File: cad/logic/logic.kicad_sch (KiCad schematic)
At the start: 32 parts, among them J1 Conn_01x02, J10 Conn_01x02, J2 Conn_01x02, J3 Conn_01x02, J4 Conn_01x02, J5 Conn_01x02, J6 Conn_01x02, J7 Conn_01x02, J8 Conn_01x02, J9 Conn_01x06, U1 74HC595, U2 TPL7407LAD, U3 TPL7407LAD, U4 TPL7407LAD

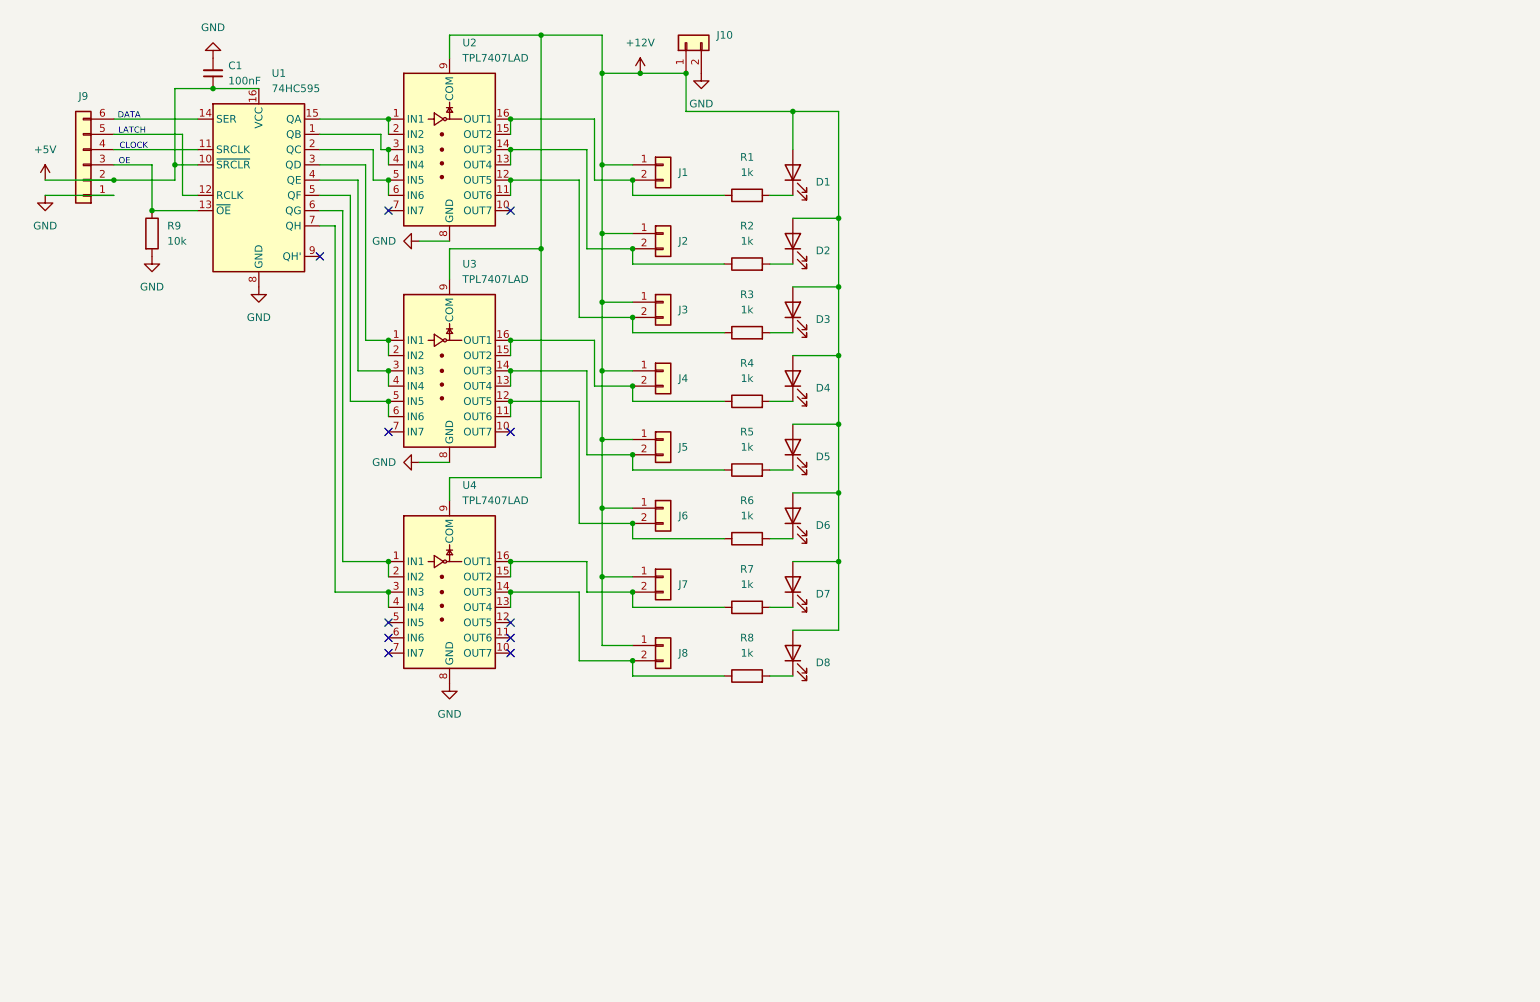
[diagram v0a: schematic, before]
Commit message: Initial design complete
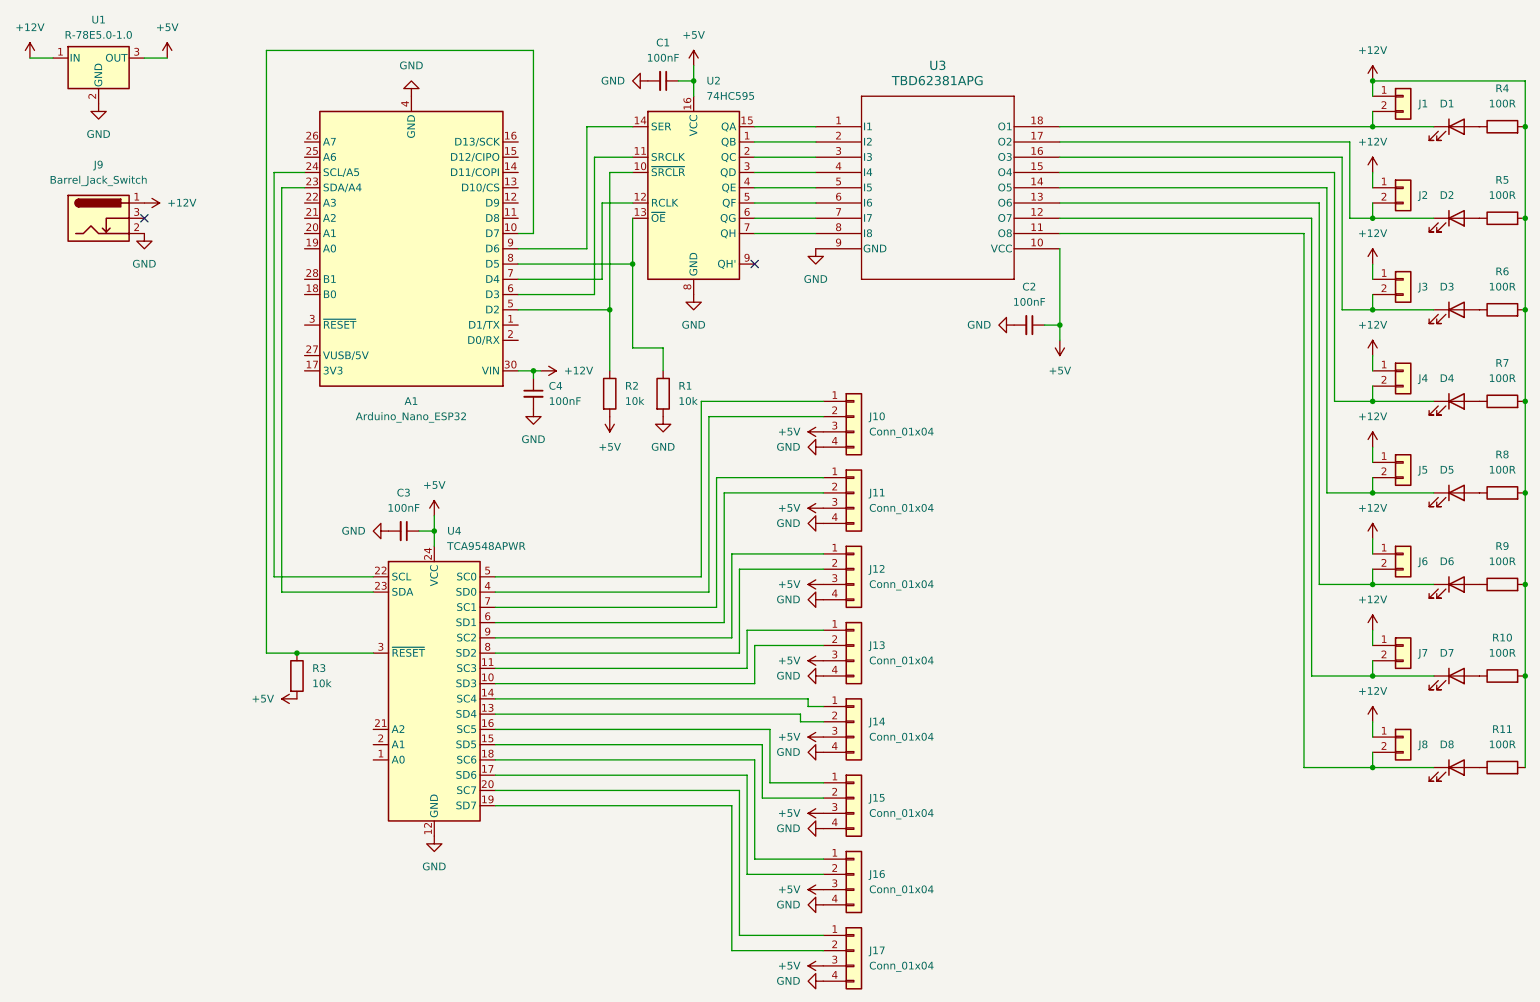
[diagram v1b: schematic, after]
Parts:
- removed J10: Conn_01x02, Connector_JST:JST_PH_B2B-PH-K_1x02_P2.00mm_Vertical, symbol Connector_Generic:Conn_01x02
- removed J9: Conn_01x06, Connector_JST:JST_PH_B6B-PH-K_1x06_P2.00mm_Vertical, symbol Connector_Generic:Conn_01x06
- removed U1: 74HC595, Package_DIP:DIP-16_W7.62mm_Socket, symbol 74xx:74HC595
- removed U2, U3, U4: TPL7407LAD, Package_SO:SOIC-16_3.9x9.9mm_P1.27mm, symbol Transistor_Array:TPL7407LAD
- added A1: Arduino_Nano_ESP32, Module:Arduino_Nano, symbol MCU_Module:Arduino_Nano_ESP32
- added C2, C3, C4: 100nF, Capacitor_THT:C_Disc_D4.7mm_W2.5mm_P5.00mm, symbol Device:C_Small
- added J10, J11, J12, J13, J14, J15, J16, J17: Conn_01x04, Connector_JST:JST_PH_B4B-PH-K_1x04_P2.00mm_Vertical, symbol Connector_Generic:Conn_01x04
- added J9: Barrel_Jack_Switch, Connector_BarrelJack:BarrelJack_Horizontal, symbol Connector:Barrel_Jack_Switch
- added R10, R11: 100R, Resistor_THT:R_Axial_DIN0207_L6.3mm_D2.5mm_P7.62mm_Horizontal, symbol Device:R
- added U1: R-78E5.0-1.0, Converter_DCDC:Converter_DCDC_RECOM_R-78E-0.5_THT, symbol Regulator_Switching:R-78E5.0-1.0
- added U2: 74HC595, Package_DIP:DIP-16_W7.62mm_Socket, symbol 74xx:74HC595
- added U3: TBD62381APG, footprints:P-DIP18-300-2p54-001_TOS, symbol watersystem:TBD62381APG
- added U4: TCA9548APWR, Package_DIP:DIP-24_18.0mmx34.29mm_W15.24mm_Socket, symbol Interface_Expansion:TCA9548APWR
- C1: footprint Capacitor_SMD:C_0805_2012Metric_Pad1.18x1.45mm_HandSolder -> Capacitor_THT:C_Disc_D4.7mm_W2.5mm_P5.00mm
- R1, R2, R3: value 1k -> 10k
- R4, R5, R6, R7, R8: value 1k -> 100R
- R9: value 10k -> 100R
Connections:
- net +12V: now also R4.2, R5.2, R6.2, R7.2, R8.2, R9.2, A1.30 (VIN), C4.1, J9.1, R10.2, R11.2, U1.1 (IN); no longer D1.2 (A), D2.2 (A), D3.2 (A), D4.2 (A), D5.2 (A), D6.2 (A), D7.2 (A), D8.2 (A)
- net +5V: now also R2.2, R3.2, C2.1, C3.1, J10.3 (Pin_3), J11.3 (Pin_3), J12.3 (Pin_3), J13.3 (Pin_3), J14.3 (Pin_3), J15.3 (Pin_3), J16.3 (Pin_3), J17.3 (Pin_3), U1.3 (OUT), U2.16 (VCC), U3.10 (VCC), U4.24 (VCC)
- net GND: now also R1.2, A1.29 (GND), A1.4 (GND), C2.2, C3.2, C4.2, J10.4 (Pin_4), J11.4 (Pin_4), J12.4 (Pin_4), J13.4 (Pin_4), J14.4 (Pin_4), J15.4 (Pin_4), J16.4 (Pin_4), J17.4 (Pin_4), J9.2, U1.2 (GND), U2.8 (GND), U3.9 (GND), U4.12 (GND); no longer R9.2
- net at D6.1 (K): now also J6.2 (Pin_2), U3.13 (O6); no longer R6.2
- net at D2.1 (K): now also J2.2 (Pin_2), U3.17 (O2); no longer R2.2
- net at R6.1: now also D3.2 (A); no longer J6.2 (Pin_2)
- net at R5.1: now also D2.2 (A); no longer J5.2 (Pin_2)
- net at J4.2 (Pin_2): now also D4.1 (K), U3.15 (O4); no longer R4.1
- net at D5.1 (K): now also J5.2 (Pin_2), U3.14 (O5); no longer R5.2
- net at R3.1: now also A1.10 (D7), U4.3 (~{RESET}); no longer J3.2 (Pin_2)
- net at R2.1: now also A1.5 (D2), U2.10 (~{SRCLR}); no longer J2.2 (Pin_2)
- net at R1.1: now also A1.8 (D5), U2.13 (~{OE}); no longer J1.2 (Pin_2)
- net at D3.1 (K): now also J3.2 (Pin_2), U3.16 (O3); no longer R3.2
- net at R9.1: now also D6.2 (A)
- net at J7.2 (Pin_2): now also D7.1 (K), U3.12 (O7); no longer R7.1
- net at J8.2 (Pin_2): now also D8.1 (K), U3.11 (O8); no longer R8.1
- net at D1.1 (K): now also J1.2 (Pin_2), U3.18 (O1); no longer R1.2
- new net: D7.2 (A), R10.1
- new net: D5.2 (A), R8.1
- new net: J13.2 (Pin_2), U4.10 (SD3)
- new net: J13.1 (Pin_1), U4.11 (SC3)
- new net: J14.2 (Pin_2), U4.13 (SD4)
- new net: J14.1 (Pin_1), U4.14 (SC4)
- new net: J15.2 (Pin_2), U4.15 (SD5)
- new net: J15.1 (Pin_1), U4.16 (SC5)
- new net: J16.2 (Pin_2), U4.17 (SD6)
- new net: J16.1 (Pin_1), U4.18 (SC6)
- new net: J17.2 (Pin_2), U4.19 (SD7)
- new net: J17.1 (Pin_1), U4.20 (SC7)
- new net: A1.24 (SCL/A5), U4.22 (SCL)
- new net: A1.23 (SDA/A4), U4.23 (SDA)
- new net: J10.2 (Pin_2), U4.4 (SD0)
- new net: J10.1 (Pin_1), U4.5 (SC0)
- new net: J11.2 (Pin_2), U4.6 (SD1)
- new net: J11.1 (Pin_1), U4.7 (SC1)
- new net: J12.2 (Pin_2), U4.8 (SD2)
- new net: J12.1 (Pin_1), U4.9 (SC2)
- new net: A1.6 (D3), U2.11 (SRCLK)
- new net: A1.7 (D4), U2.12 (RCLK)
- new net: A1.9 (D6), U2.14 (SER)
- new net: U2.15 (QA), U3.1 (I1)
- new net: U2.1 (QB), U3.2 (I2)
- new net: U2.2 (QC), U3.3 (I3)
- new net: U2.3 (QD), U3.4 (I4)
- new net: U2.4 (QE), U3.5 (I5)
- new net: U2.5 (QF), U3.6 (I6)
- new net: U2.6 (QG), U3.7 (I7)
- new net: U2.7 (QH), U3.8 (I8)
- new net: D1.2 (A), R4.1
- new net: D8.2 (A), R11.1
- new net: D4.2 (A), R7.1
- no-connect marks 11 -> 2
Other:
- note removed: "CLOCK"
- note removed: "DATA"
- note removed: "LATCH"
- note removed: "OE"
- moved on the sheet: D1, J1
